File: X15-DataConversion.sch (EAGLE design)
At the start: 26 parts, among them Y1 ECS-80-18-4X

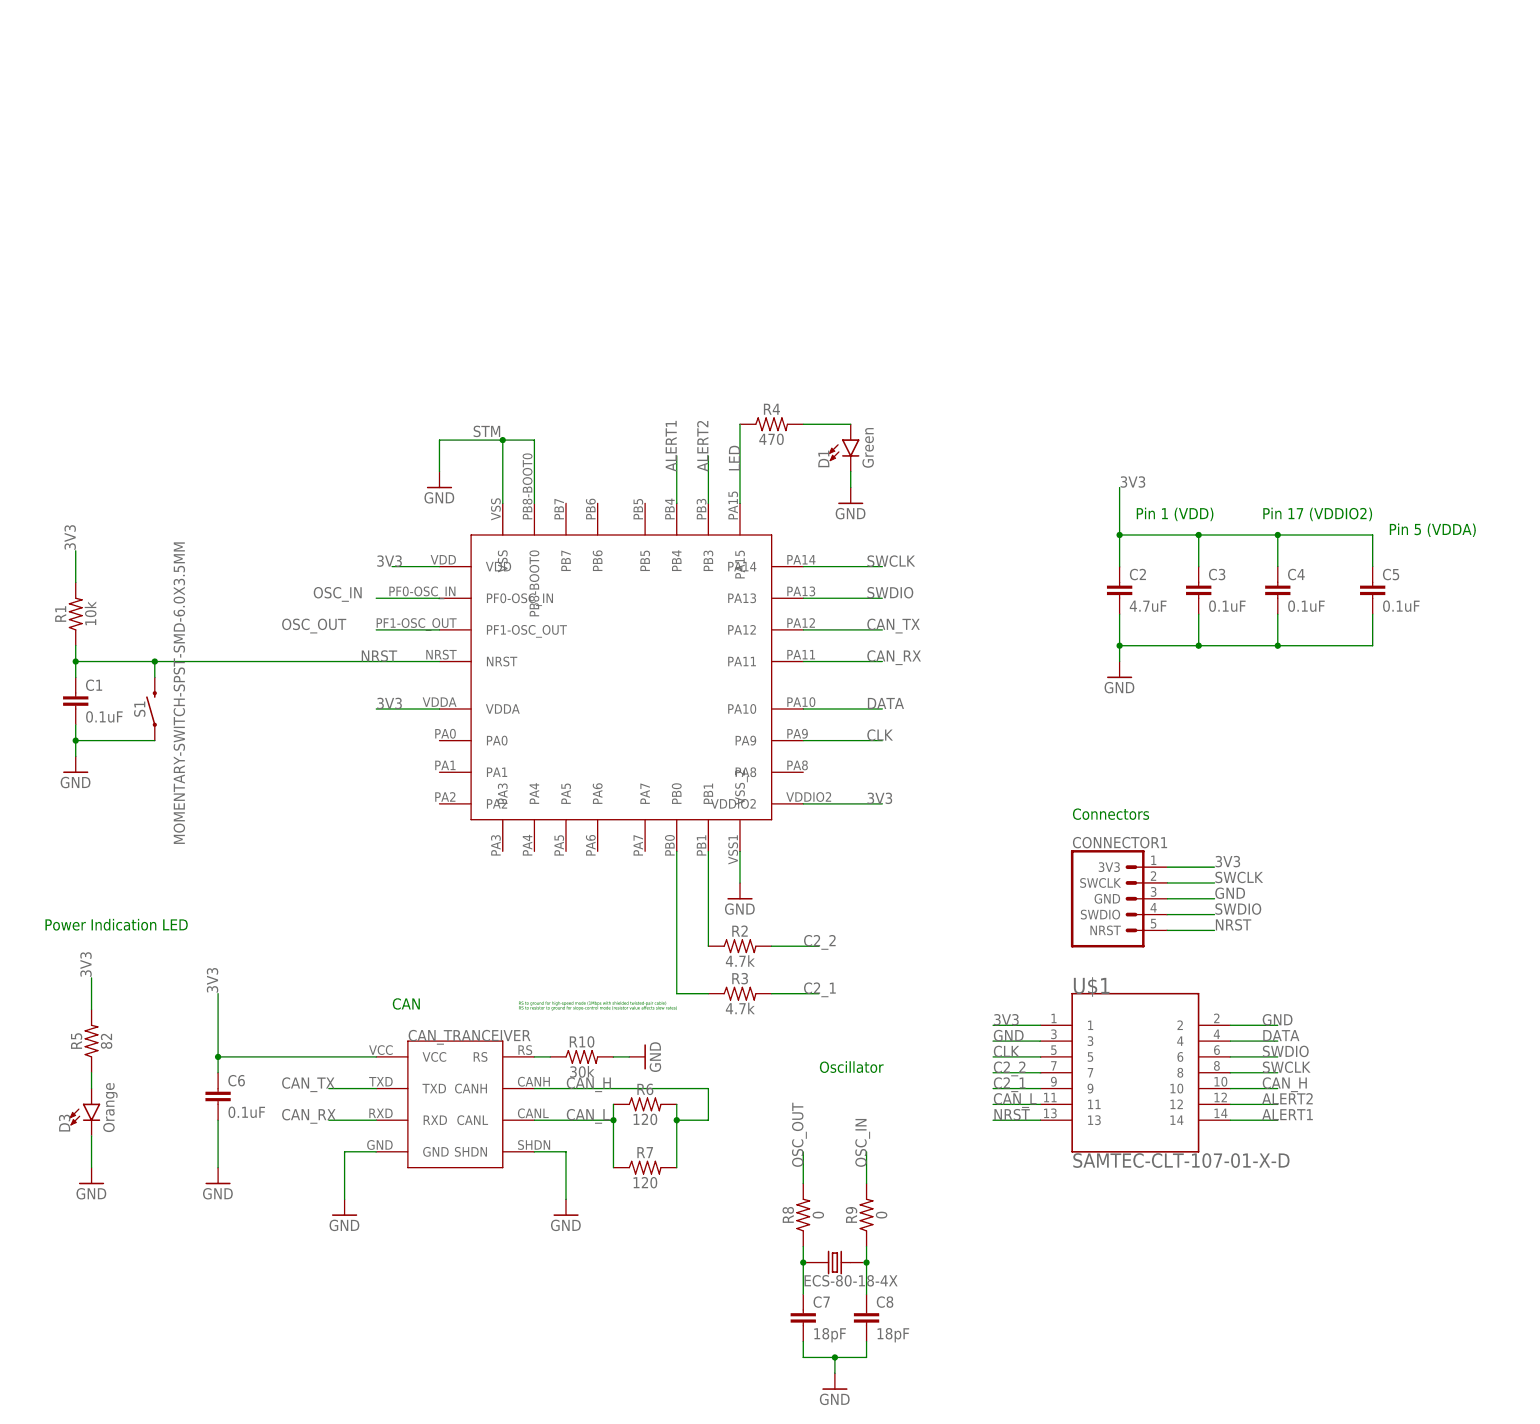
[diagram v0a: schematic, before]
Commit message: cleaning up board layout
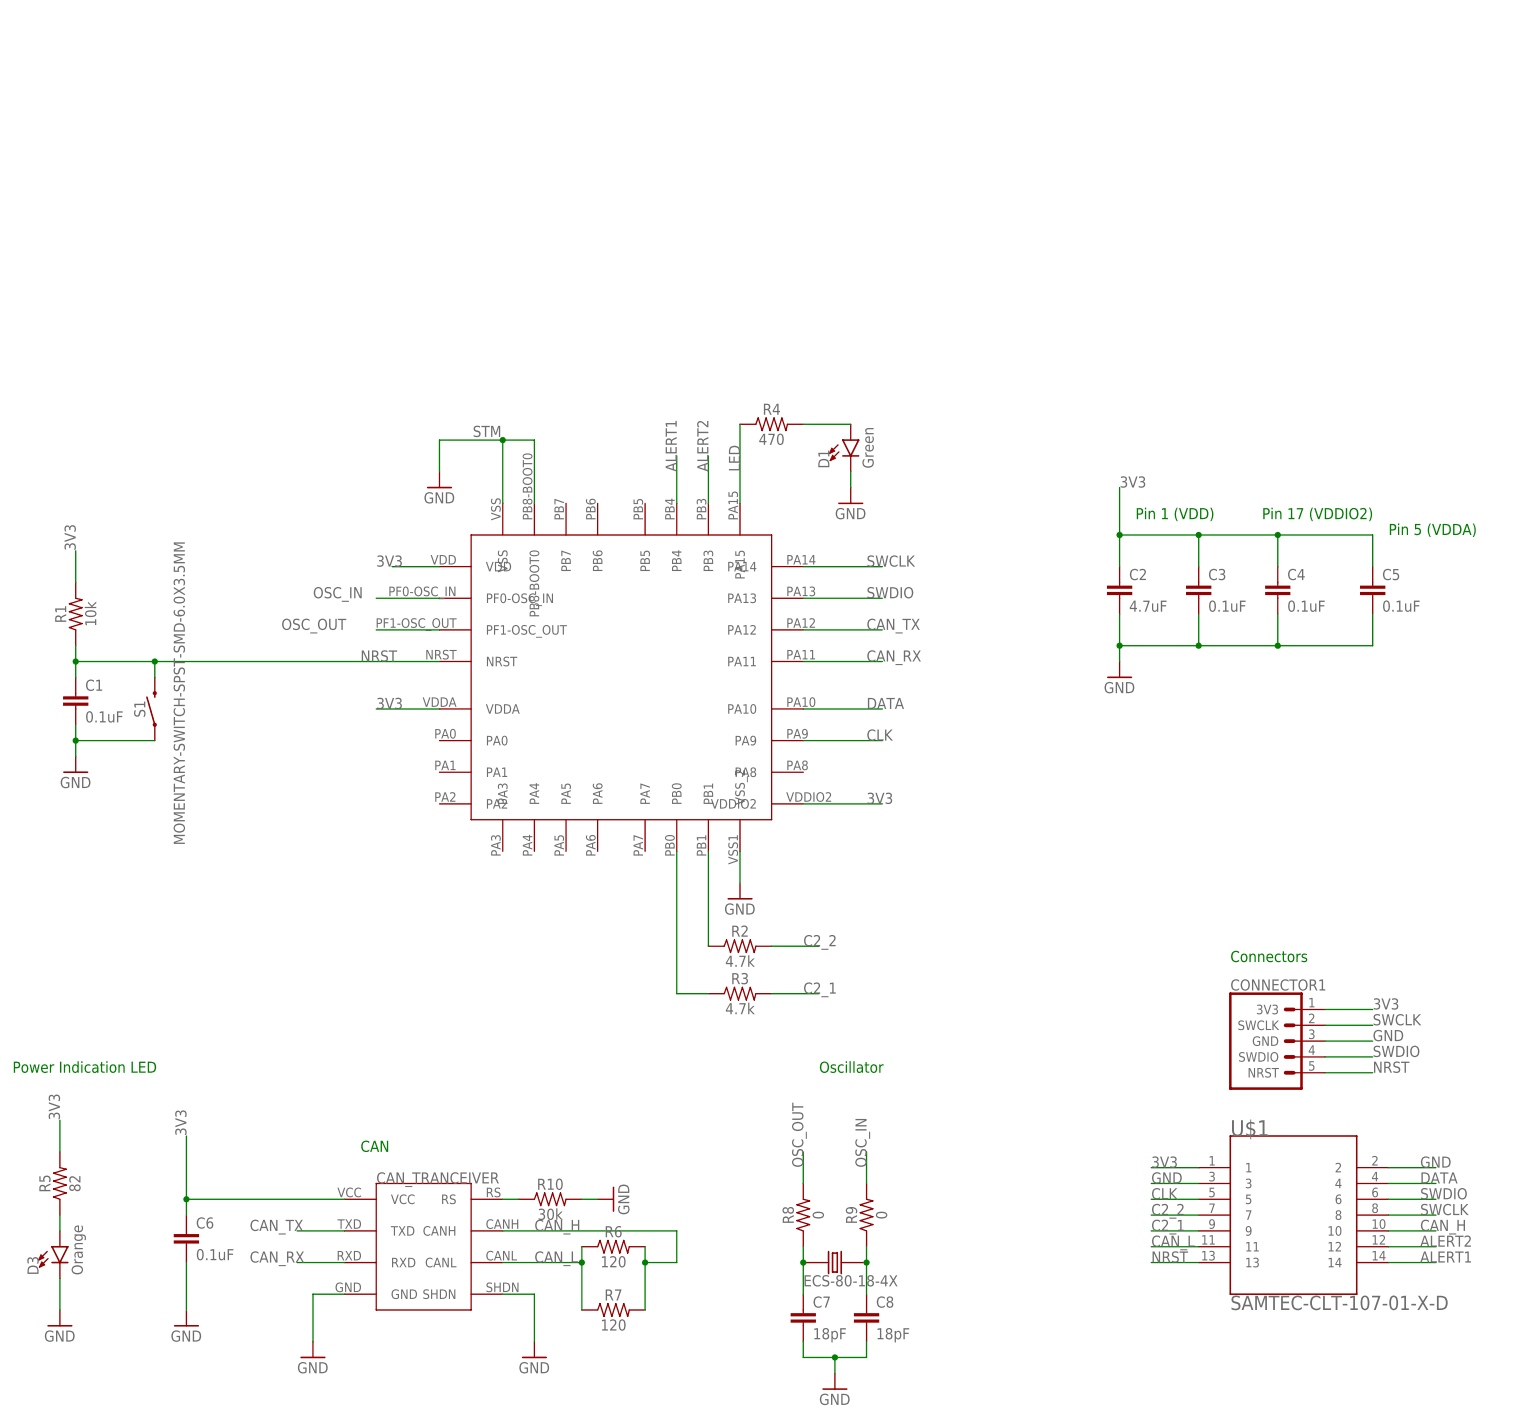
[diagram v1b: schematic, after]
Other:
- note removed: "RS to ground for high-speed mode (1Mbps with shielded twisted-pair cable) RS to resistor to ground for slope-control mode (resistor value affects slew rates)"
- moved on the sheet: C6, CAN_TRANCEIVER, CONNECTOR1, D3, R10, R5, R6, R7, U$1

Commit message: alumni review changes
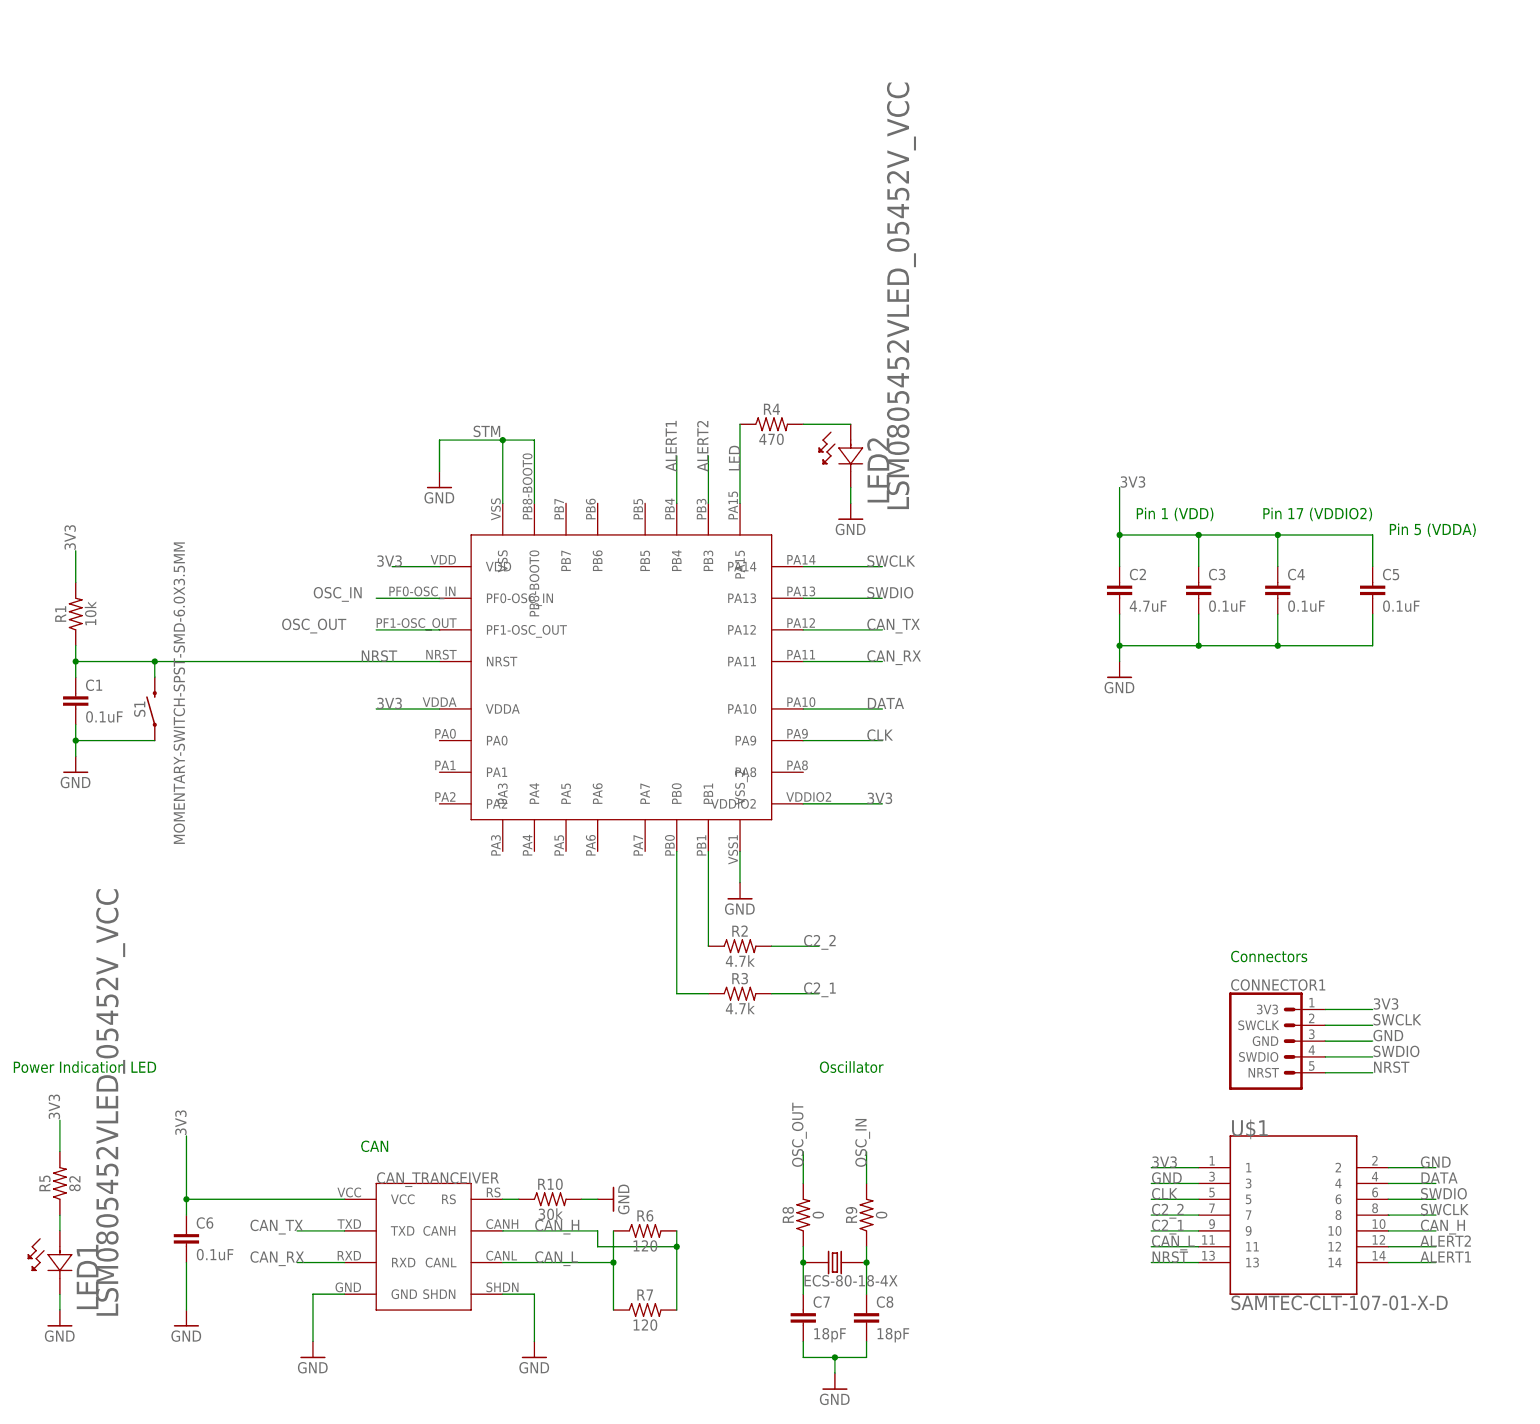
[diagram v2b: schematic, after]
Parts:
- removed D1: Green, SparkFun-LED:LED-GREEN-0603-WE
- removed D3: Orange, SparkFun-LED:LED0603
- added LED1, LED2: LSM0805452VLED_05452V_VCC, X15-Data-Conversion-Parts:LSM0805452VLED_05452V_VCC
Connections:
- net GND: now also LED1.2, LED2.2; no longer D1.C, D3.C
- net N$1: now also LED1.1; no longer D3.A
- net N$11: now also LED2.1; no longer D1.A
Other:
- moved on the sheet: R6, R7
